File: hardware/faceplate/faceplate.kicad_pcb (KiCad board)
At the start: 2 copper layers, 9.8 x 128.5 mm, 10 parts

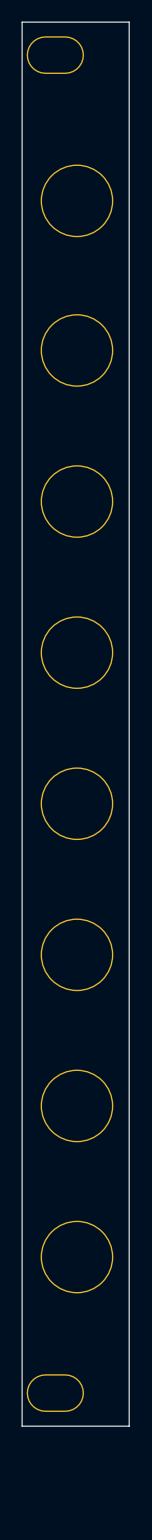
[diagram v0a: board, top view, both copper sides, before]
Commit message: New faceplate
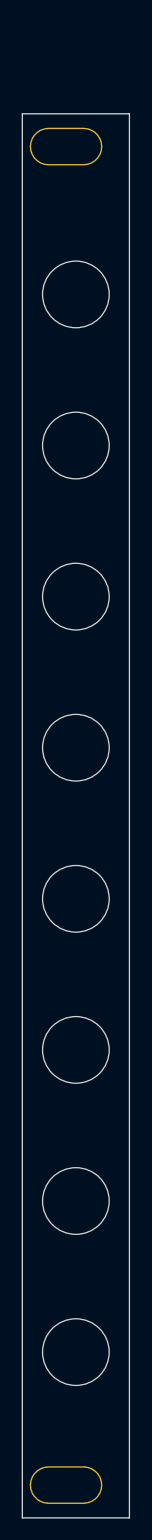
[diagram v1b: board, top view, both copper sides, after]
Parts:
- removed REF** (x8): PJ398_faceplate_hole, ModularMountingKit:PJ398_faceplate_hole
- removed REF** (x2): EuroRack_MountingHole, ModularMountingKit:EuroRack_MountingHole
- added H1: Jack 1, ModularMountingHoles:6mm_Jack, F.Cu at (54.9, 66.5)
- added H10: MountingHole, ModularMountingHoles:Eurorack_mounting_hole, F.Cu at (54.0, 175.5)
- added H2: Jack 2, ModularMountingHoles:6mm_Jack, F.Cu at (54.9, 80.4)
- added H3: Jack 3, ModularMountingHoles:6mm_Jack, F.Cu at (54.9, 94.2)
- added H4: Jack 4, ModularMountingHoles:6mm_Jack, F.Cu at (54.9, 108.0)
- added H5: Jack 5, ModularMountingHoles:6mm_Jack, F.Cu at (54.9, 121.8)
- added H6: Jack 6, ModularMountingHoles:6mm_Jack, F.Cu at (54.9, 135.7)
- added H7: Jack 7, ModularMountingHoles:6mm_Jack, F.Cu at (54.9, 149.5)
- added H8: Jack 8, ModularMountingHoles:6mm_Jack, F.Cu at (54.9, 163.3)
- added H9: MountingHole, ModularMountingHoles:Eurorack_mounting_hole, F.Cu at (54.0, 53.0)
